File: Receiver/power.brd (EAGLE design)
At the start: 31.8 x 33 mm, 22 parts, among them IC1 7805TV

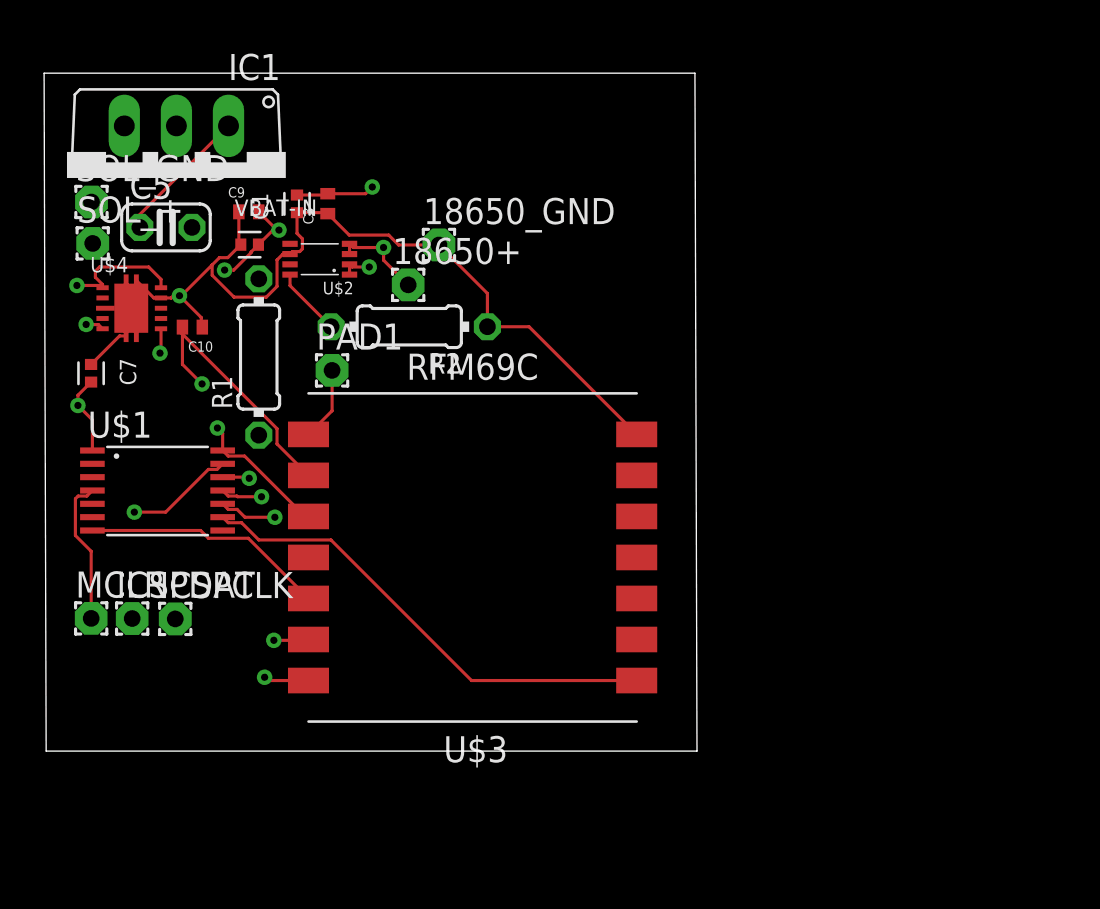
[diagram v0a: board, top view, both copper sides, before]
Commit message: recently printed version, transfer to test on windows mplab
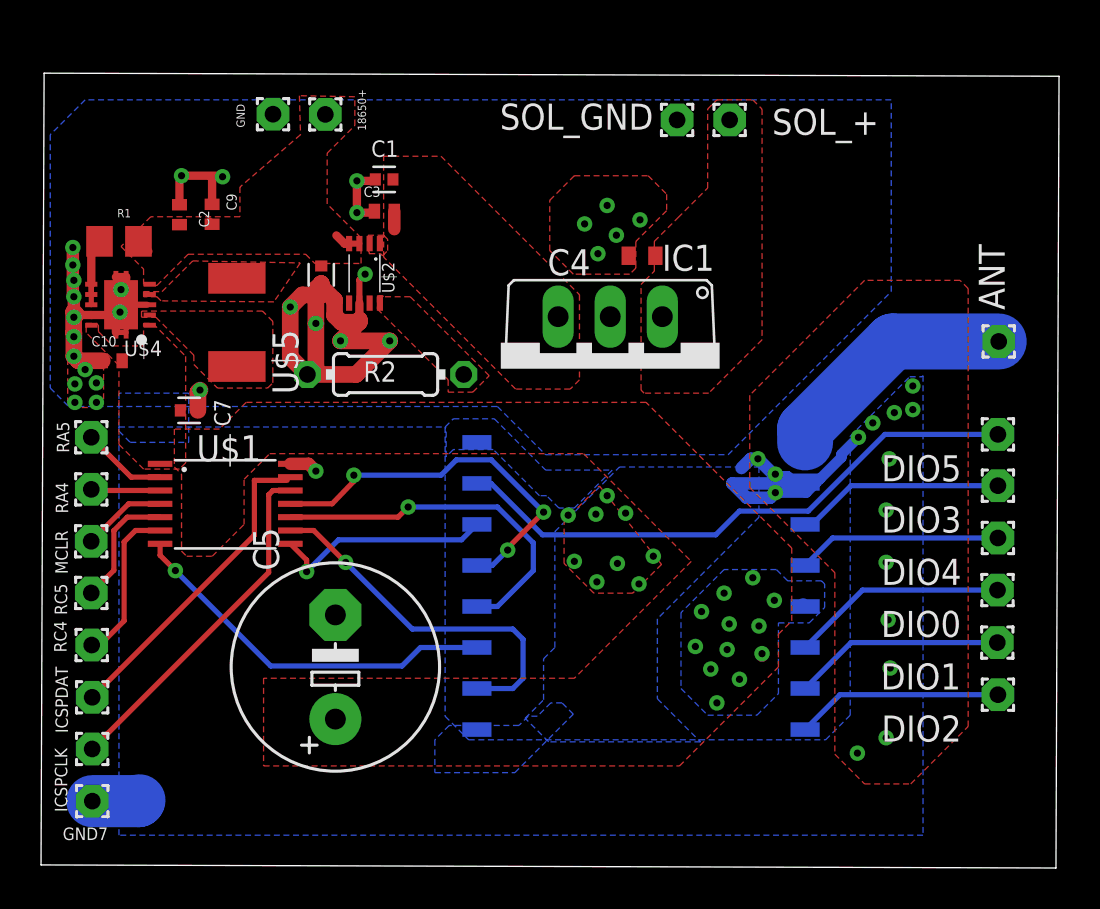
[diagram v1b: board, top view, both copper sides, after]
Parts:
- removed 18650_GND, PAD1: (no value), wirepad:1,6/0,8
- added ANT, DIO0, DIO1, DIO2, DIO3, DIO4, DIO5, GND, GND7, RA4, RA5, RC4, RC5: (no value), wirepad:1,6/0,8
- added C2: 1uf, UMK105CBJ105KV-F:CAPC1005X70N
- added C4: (no value), rcl:C0402
- added U$5: SRP0510-2R2K, SRP0510-2R2K :SRP0510-2R2K
- C5: value .33uf -> 330uf; device rcl:C025-024X044 -> rcl:E5-10,5
- R1: device rcl:0204/7 -> rcl:R0805
- U$3: value RFM69C -> RFM69HCW; device RFM69C:RFM69C -> RFM69C:RFM69HCW
- moved SOL_+ 31.6 mm to (33.3, 30.8)
- moved SOL_GND 28.8 mm to (30.8, 30.8)
- moved IC1 23.1 mm to (27.5, 18.6)
- moved C5 23.0 mm to (14.1, 4.10), turned to 90 degrees
- moved 18650+ 9.24 mm to (13.6, 31.0)
- moved R1 8.85 mm to (3.55, 24.9), turned to 0 degrees
- moved U$3 8.33 mm to (29.0, 8.05), flipped to the bottom
- moved ICSPCLK 7.52 mm to (2.24, 0.10)
- moved C7 5.11 mm to (6.97, 16.6), turned to 180 degrees
- moved C1 4.41 mm to (16.5, 27.9), turned to 0 degrees
- moved ICSPDAT 4.31 mm to (2.24, 2.62)
- moved C10 4.24 mm to (3.22, 19.0), turned to 0 degrees
- moved VBAT-IN 3.79 mm to (13.4, 23.2), turned to 90 degrees
- moved MCLR 3.76 mm to (2.20, 10.2)
- moved U$1 3.36 mm to (8.73, 12.0)
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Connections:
- removed net MISO: U$1.9, U$3.8
- new net N$15: DIO1.1, U$3.DIO1
- new net N$16: DIO0.1, U$3.DIO0
- new net N$17: DIO4.1, U$3.DIO4
- new net N$18: DIO3.1, U$3.DIO3
- new net N$19: ANT.1, U$3.ANT
- new net N$20: DIO5.1, U$3.DIO5
- new net N$21: U$4.4, U$5.P$1
- new net N$22: U$4.2, U$5.P$2
- new net N$3: RA4.1, U$1.3
- new net N$6: RA5.1, U$1.2
- new net N$7: RC5.1, U$1.5
- new net N$8: RC4.1, U$1.6
- new net N$9: DIO2.1, U$3.DIO2
- new net SOL_IN: C4.1, IC1.1, SOL_+.1
- net GND: now also C2.1, C4.2, C5.-, GND.1, GND7.1, U$3.GND@1, U$3.GND@2, U$3.GND@3; no longer 18650_GND.1, C5.2, U$3.14, U$3.3
- net MOSI: now also U$3.MOSI; no longer U$3.5
- net N$1: now also U$1.9, U$3.MISO; no longer C5.1, IC1.1, SOL_+.1
- net N$2: now also R1.1; no longer R1.2
- net N$4: now also U$1.8, U$3.RESET; no longer PAD1.1, U$3.1
- net SCK: now also U$3.SCK; no longer U$3.6
- net SS: now also U$3.NSS; no longer U$3.7
- net VBAT-IN: now also C2.2, R1.2; no longer R1.1
- net VOUT: now also C5.+, U$3.3.3V; no longer U$3.2
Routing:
- net VOUT: track 35.6 -> 0.24 mm, vias 3 -> 12
- net VBAT-IN: track 32.7 -> 2.72 mm, vias 4 -> 0
- net N$20: track 0.00 -> 28.5 mm
- net MISO: track 23.5 -> 0.00 mm
- net VIN-5V: track 23.7 -> 1.41 mm, vias 2 -> 0
- net N$19: track 0.00 -> 11.9 mm
- net N$16: track 0.00 -> 10.5 mm
- net N$15: track 0.00 -> 10.3 mm
- net N$18: track 0.00 -> 10.2 mm
- net N$9: track 0.00 -> 10.1 mm
- net N$17: track 0.00 -> 9.96 mm
- net N$1: track 9.36 -> 17.9 mm, vias 0 -> 1
- net N$8: track 0.00 -> 7.90 mm
- net N$12: track 9.67 -> 17.1 mm, vias 1 -> 0
- net N$4: track 3.60 -> 10.9 mm, vias 0 -> 1
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- added copper zone on layer 1, net GND
- added copper zone on layer 16, net GND
- added copper zone on layer 1, net N$21
- added copper zone on layer 1, net N$22
- added copper zone on layer 1, net N$5
- added copper zone on layer 1, net SOL_IN
- added copper zone on layer 1, net VBAT-IN
- added copper zone on layer 1, net VIN-5V
- added copper zone on layer 1, net VOUT
- added copper zone on layer 16, net VOUT
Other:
- board size 31.8 x 33 mm -> 49.6 x 38.8 mm
